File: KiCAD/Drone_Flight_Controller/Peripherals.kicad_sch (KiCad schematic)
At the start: 57 parts, among them J1 XT60, J2 0.5mΩ high side shunt, Q1 2N2222A, U1 74AHC1G125, U2 74AHC1G125, U3 74AHC1G125, U4 74AHC1G125, U9 INA195

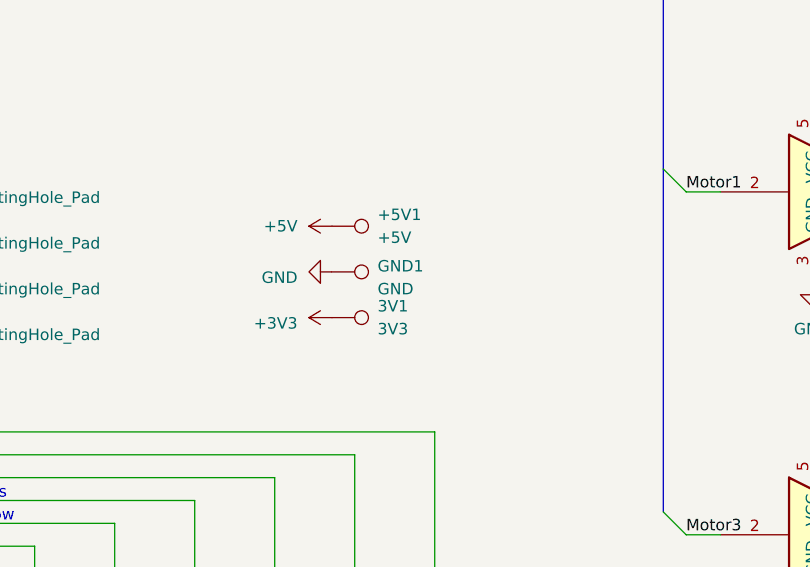
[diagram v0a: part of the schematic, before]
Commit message: Revision
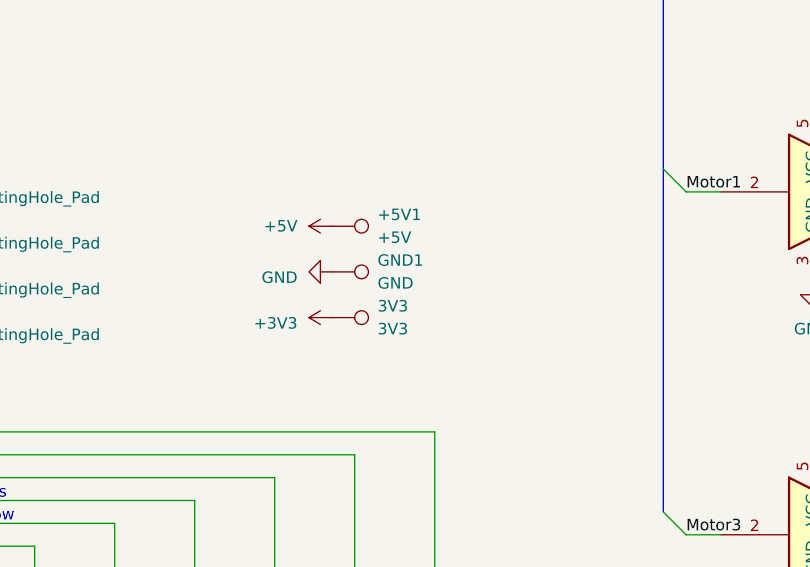
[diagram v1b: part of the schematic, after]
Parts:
- renumbered 3V1 to 3V3
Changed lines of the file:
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@@
 		(dnp no)
 		(fields_autoplaced yes)
-		(property "Reference" "3V1"
+		(property "Reference" "3V3"
 			(at 93.98 120.6499 90)
 			(effects
@@
 			(project "Drone_Flight_Controller"
 				(path "/51ab9491-7068-4b24-bb38-47a0c739796e/a1832adb-c070-4778-a5ef-97ea378c06da"
-					(reference "3V1")
+					(reference "3V3")
 					(unit 1)
 				)
@@
 		(fields_autoplaced yes)
 		(property "Reference" "GND1"
-			(at 93.98 116.205 90)
+			(at 93.98 115.5699 90)
 			(effects
 				(font
@@
 		)
 		(property "Value" "GND"
-			(at 93.98 118.745 90)
-			(effects
-				(font
+			(at 93.98 118.1099 90)
+			(effects
+				(font
